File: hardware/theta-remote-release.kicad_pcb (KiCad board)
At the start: 2 copper layers, 48 x 39 mm, 21 parts, among them P1 Li-Po Battery, SW1 POWER, SW2 PUSH-SW, U1 AE-FT234X, U2 MCP73831, U3 ESP-WROOM-02, U4 TPS63000

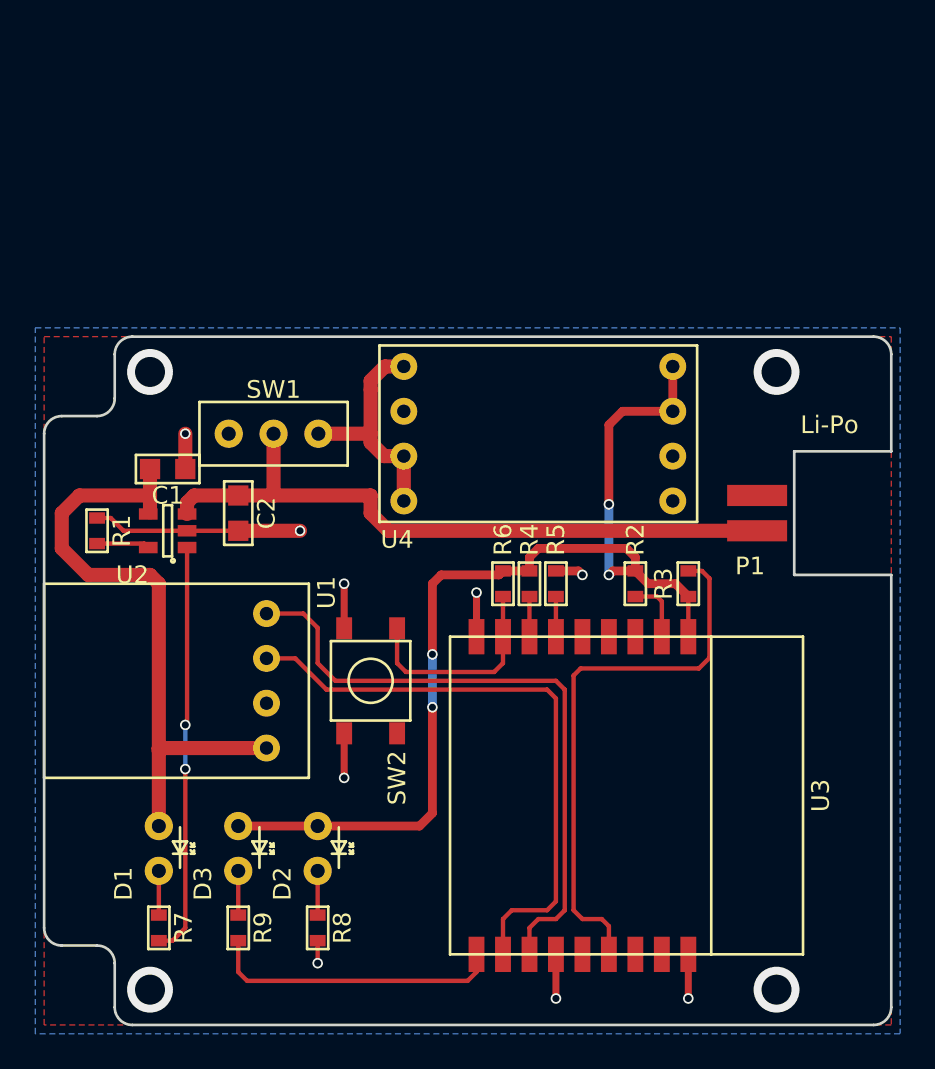
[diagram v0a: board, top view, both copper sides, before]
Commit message: add 1.0.0
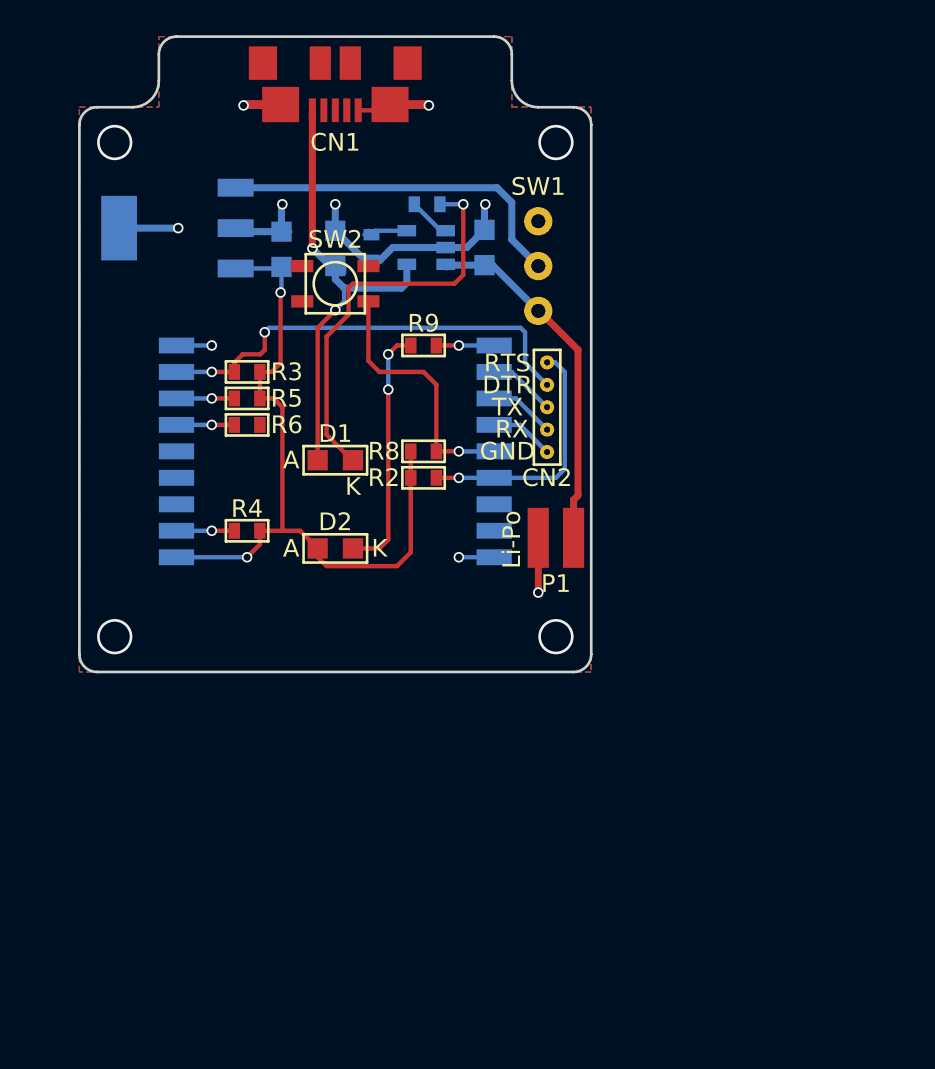
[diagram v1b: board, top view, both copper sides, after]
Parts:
- removed D3: STATUS, theta-remote-release:LED
- removed U4: TPS63000, theta-remote-release:TPS63000
- added C3: 4.7uF, theta-remote-release:SMD2012, B.Cu at (135.4, 81.0)
- added CN1: ZX62R-B-5P, theta-remote-release:ZX62R-B-5P, F.Cu at (138.5, 70.5)
- added CN2: DEBUG, theta-remote-release:Debug, F.Cu at (150.5, 90.0)
- C1, C2: value 4.7μF -> 4.7uF; moved to B.Cu
- D1: value CHARGE -> CHG; footprint theta-remote-release:LED -> theta-remote-release:SMD2012_LED
- D2: value POWER -> STAT; footprint theta-remote-release:LED -> theta-remote-release:SMD2012_LED
- P1: value Li-Po Battery -> Li-Po 3.7V; footprint theta-remote-release:PH-2P-TOP-SIDE -> theta-remote-release:Li-Po
- R1: value 2kΩ -> 10k; moved to B.Cu
- R2, R3, R4, R5: value 10kΩ -> 10k
- R6: value 4.7kΩ -> 10k
- R7: value 470Ω -> 100; moved to B.Cu
- R8: value 470Ω -> 10k
- R9: value 470Ω -> 100
- SW1: footprint theta-remote-release:SS12D01G4 -> theta-remote-release:ESP2020
- SW2: value PUSH-SW -> SHUTTER; footprint theta-remote-release:PUSH-SW -> theta-remote-release:TVAF17-WEC-R
- U1: value AE-FT234X -> MCP73831; footprint theta-remote-release:AE-FT234X -> TO_SOT_Packages_SMD:SOT-23-5; moved to B.Cu
- U2: value MCP73831 -> ESP-WROOM-02; footprint TO_SOT_Packages_SMD:SOT-23-5 -> theta-remote-release:esp-wroom-02; moved to B.Cu
- U3: value ESP-WROOM-02 -> MCP1825S-3002E/DB; footprint theta-remote-release:esp-wroom-02 -> TO_SOT_Packages_SMD:SOT-223; moved to B.Cu
- moved R7 43.7 mm to (143.7, 78.5), turned to 180 degrees
- moved U3 35.7 mm to (129.6, 79.8)
- moved R9 34.6 mm to (143.5, 86.5), turned to 0 degrees
- moved U1 28.3 mm to (143.7, 81.0), turned to 180 degrees
- moved R3 27.7 mm to (133.5, 88.0), turned to 180 degrees
- moved R8 27.7 mm to (143.5, 92.5), turned to 0 degrees
- moved D1 24.2 mm to (138.5, 93.0), turned to 180 degrees
- moved SW2 22.6 mm to (138.5, 83.0), turned to 180 degrees
- moved R1 22.3 mm to (140.6, 81.0), turned to 90 degrees
- moved C2 20.5 mm to (146.9, 81.0), turned to 90 degrees
- moved R5 20.4 mm to (133.5, 89.5), turned to 180 degrees
- moved SW1 17.8 mm to (150.0, 82.0), turned to 270 degrees
- moved R6 17.1 mm to (133.5, 91.0), turned to 180 degrees
- moved D2 17.0 mm to (138.5, 98.0), turned to 180 degrees
- moved R4 16.3 mm to (133.5, 97.0), turned to 180 degrees
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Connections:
- D2 pad 2: +3V3 -> +3V
- R2 pad 1: +3V3 -> +3V
- R2 pad 2: Net-(R2-Pad2) -> Net-(CN2-Pad1)
- R3 pad 1: +3V3 -> +3V
- R3 pad 2: Net-(R3-Pad2) -> Net-(CN2-Pad2)
- R4 pad 1: +3V3 -> +3V
- R5 pad 1: Net-(R5-Pad1) -> +3V
- R5 pad 2: GND -> Net-(R5-Pad2)
- R6 pad 1: +3V3 -> GND
- R6 pad 2: /IO0 -> Net-(R6-Pad2)
- R7 pad 2: /STAT -> /CHG
- R8 pad 1: Net-(D2-Pad1) -> +3V
- R8 pad 2: GND -> /IO5
- R9 pad 1: Net-(D3-Pad1) -> Net-(D2-Pad1)
- SW1 pad 2: Net-(C2-Pad1) -> Net-(SW1-Pad2)
- SW1 pad 3: +BATT -> Net-(C2-Pad1)
- SW2 pad 1: /IO0 -> /IO5
- U1 pad 1: +5V -> /CHG
- U1 pad 3: Net-(U1-Pad3) -> Net-(C2-Pad1)
- U1 pad 4: Net-(U1-Pad4) -> +5V
- U2 pad 1: /STAT -> +3V
- U2 pad 2: GND -> Net-(R4-Pad2)
- U2 pad 3: Net-(C2-Pad1) -> (no net)
- U2 pad 4: +5V -> (no net)
- U2 pad 5: Net-(R1-Pad2) -> (no net)
- U3 pad 1: +3V3 -> Net-(SW1-Pad2)
- U3 pad 2: Net-(R2-Pad2) -> GND
- U3 pad 3: (no net) -> +3V
- U3 pad 4: (no net) -> GND
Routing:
- net +3V3: track 60.5 -> 0.00 mm, vias 4 -> 0
- net +3V: track 0.00 -> 42.4 mm, vias 0 -> 2
- net Net-(U1-Pad4): track 36.4 -> 0.00 mm
- net Net-(U1-Pad3): track 34.8 -> 0.00 mm
- net Net-(R3-Pad2): track 31.5 -> 0.00 mm
- net Net-(CN2-Pad2): track 0.00 -> 25.3 mm, vias 0 -> 2
- net /STAT: track 23.4 -> 0.00 mm, vias 2 -> 0
- net Net-(D1-Pad1): track 2.51 -> 23.1 mm, vias 0 -> 1
- net Net-(SW1-Pad2): track 0.00 -> 20.2 mm
- net Net-(C2-Pad1): track 38.0 -> 20.3 mm
- net /IO5: track 0.00 -> 15.6 mm, vias 0 -> 1
- net Net-(CN2-Pad1): track 0.00 -> 15.0 mm, vias 0 -> 1
- net +BATT: track 13.4 -> 0.00 mm
- net /IO4: track 16.7 -> 3.28 mm, vias 0 -> 1
- net Net-(D2-Pad1): track 2.51 -> 14.2 mm, vias 0 -> 2
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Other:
- board size 48 x 39 mm -> 29 x 36 mm
